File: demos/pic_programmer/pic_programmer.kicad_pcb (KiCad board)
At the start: 2 copper layers, 68 parts, among them J1 DB9-FEMAL, P1 CONN_2, P2 SUPP28, P3 SUPP40, Q1 BC237, Q2 BC307, Q3 BC307, U1 24Cxx, U2 74HC125, U3 7805, U4 LT1373, U5 PIC_18_PINS, U6 PIC_8_PINS

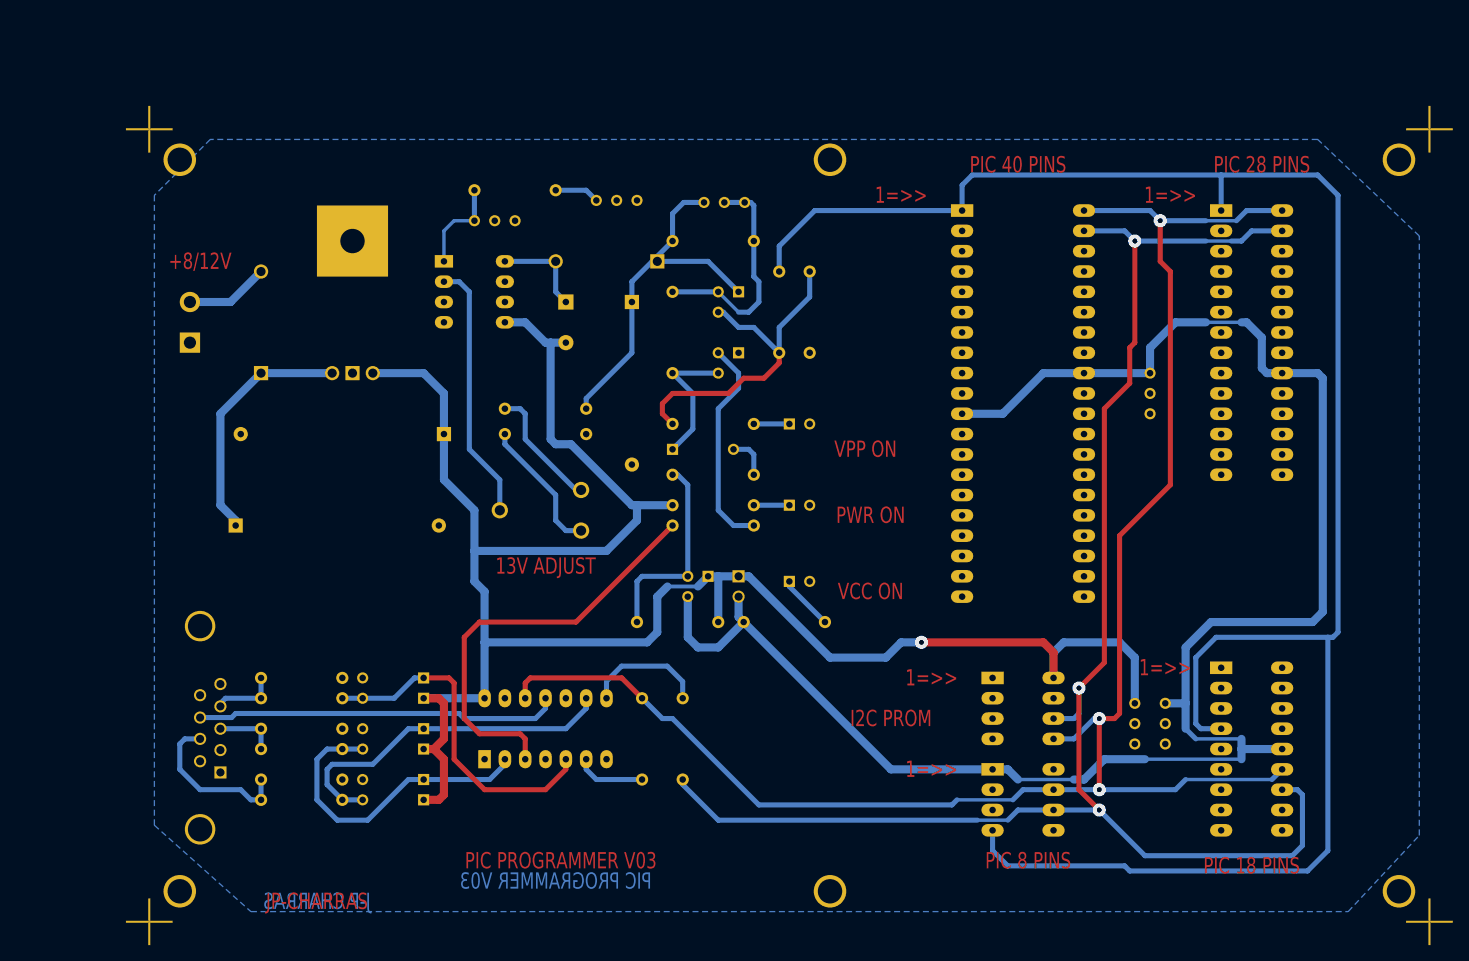
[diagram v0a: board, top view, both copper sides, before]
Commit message: Imported Upstream version 4.0.0~rc1
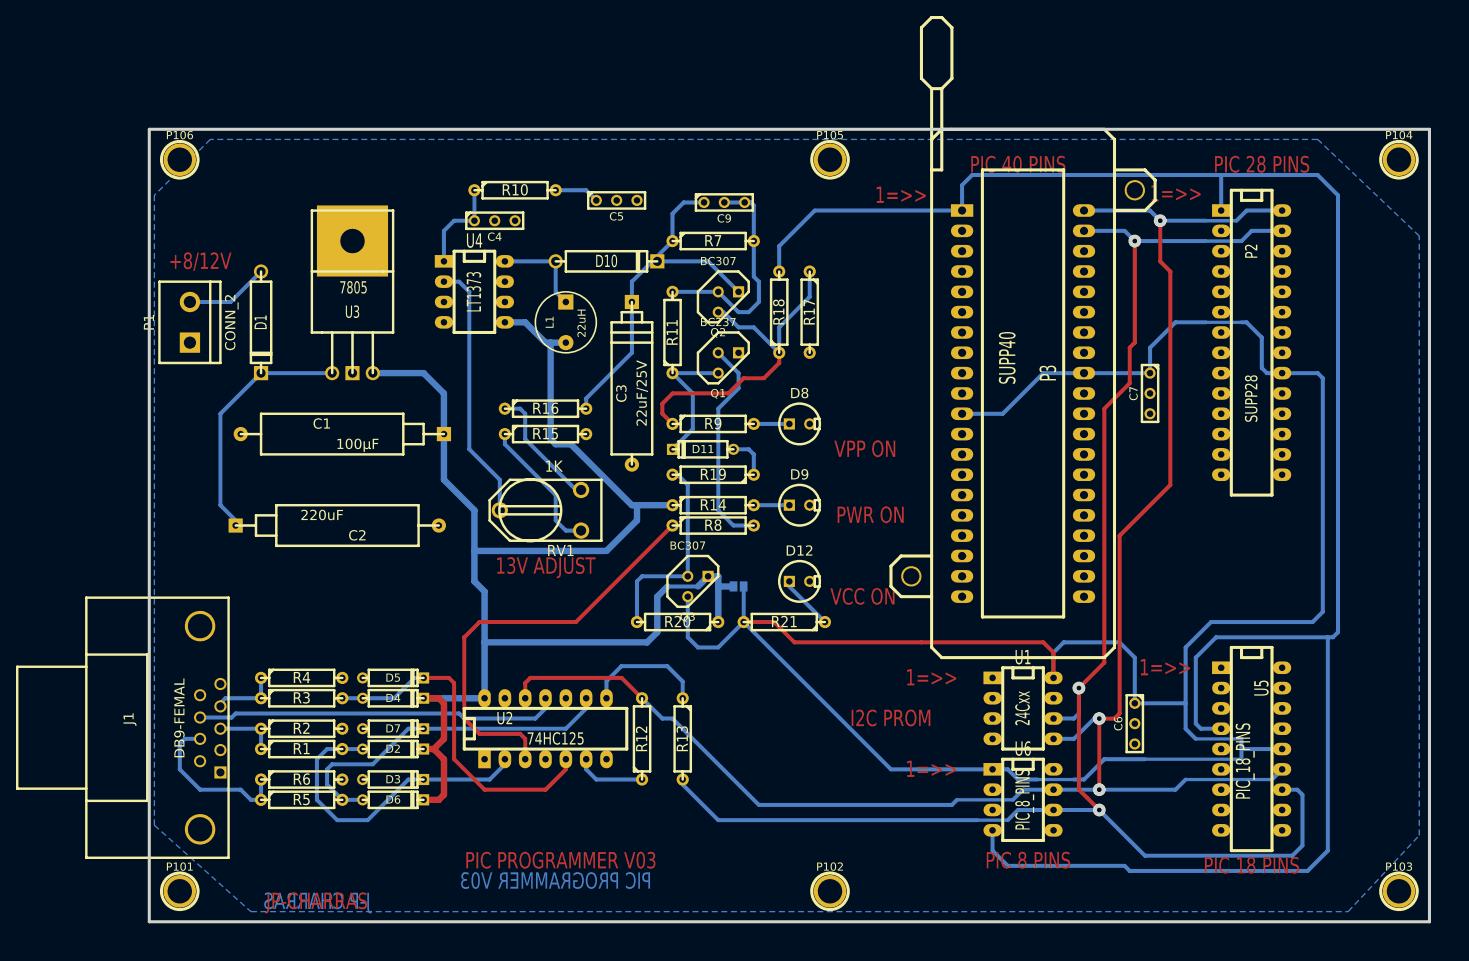
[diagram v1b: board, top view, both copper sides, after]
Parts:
- removed 1PIN (x6): P***, 1pin
- removed C8: 100nF, C1-1
- removed MIRE (x4): *, MIRE
- added P101: CONN_1, footprints:1pin-4, F.Cu at (77.5, 135.9)
- added P102: CONN_1, footprints:1pin-4, F.Cu at (158.8, 135.9)
- added P103: CONN_1, footprints:1pin-4, F.Cu at (229.9, 135.9)
- added P104: CONN_1, footprints:1pin-4, F.Cu at (229.9, 44.5)
- added P105: CONN_1, footprints:1pin-4, F.Cu at (158.8, 44.5)
- added P106: CONN_1, footprints:1pin-4, F.Cu at (77.5, 44.5)
- C1: value 100uF -> 100µF; footprint CP10 -> discret:CP10
- C2: footprint CP10 -> discret:CP10
- C3: footprint CP8 -> discret:CP8
- C4, C5, C6, C7, C9: footprint C1-1 -> discret:C1-1
- D1, D10: footprint D5 -> discret:D5
- D11, D2, D3, D4, D5, D6, D7: footprint D3 -> discret:D3
- D12, D8, D9: footprint LEDV -> discret:LEDV
- J1: footprint DB9FC -> connect:DB9FC
- JP1: footprint PIN_ARRAY_2X1 -> connect:GS2; moved to B.Cu
- L1: footprint INDUCTOR_V -> inductors:INDUCTOR_V
- P1: footprint bornier2 -> connect:bornier2
- P2: footprint 28DIP-ELL300 -> dip_sockets:DIP-28__300_ELL
- P3: footprint 40DIP-ELL600 -> sockets:40tex-Ell600
- Q1, Q2, Q3: footprint TO92 -> discret:TO92
- R1, R10, R11, R12, R13, R14, R15, R16, R17, R18, R19, R2, R20, R21, R3, R4, R5, R6, R7, R8, R9: footprint R4 -> discret:R4
- RV1: footprint RV2X4 -> discret:RV2X4
- U1, U4, U6: footprint 8DIP-ELL300 -> dip_sockets:DIP-8__300_ELL
- U2: footprint 14DIP-ELL300 -> dip_sockets:DIP-14__300_ELL
- U3: footprint LM78XX -> discret:LM78XX
- U5: footprint 18DIP-ELL300 -> dip_sockets:DIP-18__300_ELL
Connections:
- net /PC-DATA-IN renamed /CTS
- net /VPP/MCLR renamed /pic_sockets/VPP-MCLR
- net /VPP_ON renamed /TXD
- net /pic_sockets.sch/CLOCK-RB6 renamed /pic_sockets/CLOCK-RB6
- net /pic_sockets.sch/DATA-RB7 renamed /pic_sockets/DATA-RB7
- C6 pad 1: VCC -> /pic_sockets/VCC_PIC
- C7 pad 1: /pic_sockets.sch/VCC_PIC -> /pic_sockets/VCC_PIC
- JP1 pad 2: /pic_sockets.sch/VCC_PIC -> /pic_sockets/VCC_PIC
- P2 pad 20: /pic_sockets.sch/VCC_PIC -> /pic_sockets/VCC_PIC
- P3 pad 11: /pic_sockets.sch/VCC_PIC -> /pic_sockets/VCC_PIC
- P3 pad 32: /pic_sockets.sch/VCC_PIC -> /pic_sockets/VCC_PIC
- Q3 pad 3: /pic_sockets.sch/VCC_PIC -> /pic_sockets/VCC_PIC
- R21 pad 2: /pic_sockets.sch/VCC_PIC -> /pic_sockets/VCC_PIC
- U1 pad 8: VCC -> /pic_sockets/VCC_PIC
- U5 pad 14: /pic_sockets.sch/VCC_PIC -> /pic_sockets/VCC_PIC
- U6 pad 1: /pic_sockets.sch/VCC_PIC -> /pic_sockets/VCC_PIC
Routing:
- net /pic_sockets/VCC_PIC: track 0.00 -> 290.3 mm
- net /pic_sockets.sch/VCC_PIC: track 221.6 -> 0.00 mm
- net VCC: track 252.2 -> 183.3 mm, vias 1 -> 0
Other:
- board outline added: 160 x 99.1 mm
- net class Default: clearance 0.254 -> 0.25; trace_width 0.254 -> 0.5; via_dia 0.889 -> 1.6; via_drill 0.635 -> 0.6
- net class POWER added: clearance 0.28, trace_width 0.8, via_dia 1.6, via_drill 0.6
- rule pad_to_mask_clearance: 0.2 -> 0.1
- rule trace_clearance: 0.254 -> 0.25
